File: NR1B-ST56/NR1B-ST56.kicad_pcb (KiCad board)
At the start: 4 copper layers, 70.5 x 134 mm, 34 parts, among them J1 0.1" Female Long Tail, J2 0.1" Female Long Tail, J3 Conn_01x02, U1 S29GL01GP, U2 DG419LDY, U3 OPA2189ID, U4 NCV7800, X1 NUCLEO144-ZIO

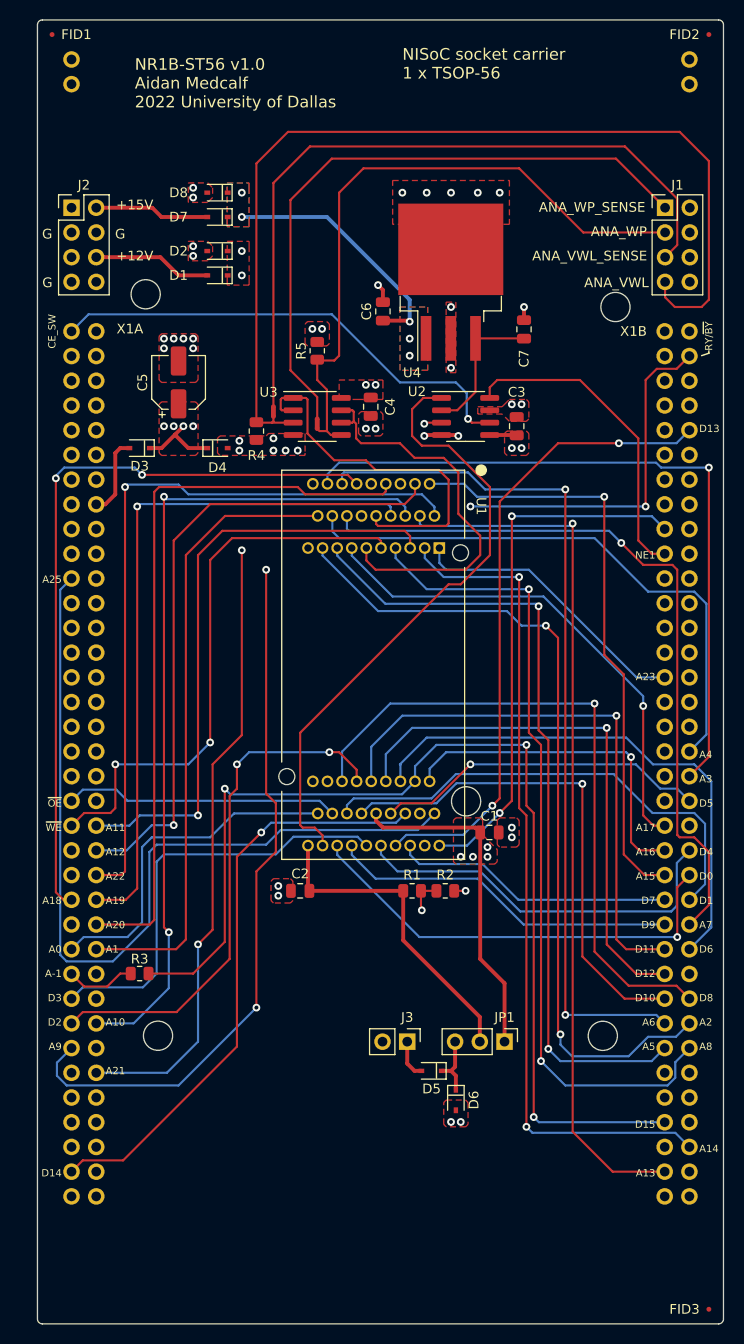
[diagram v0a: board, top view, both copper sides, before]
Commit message: Many updates
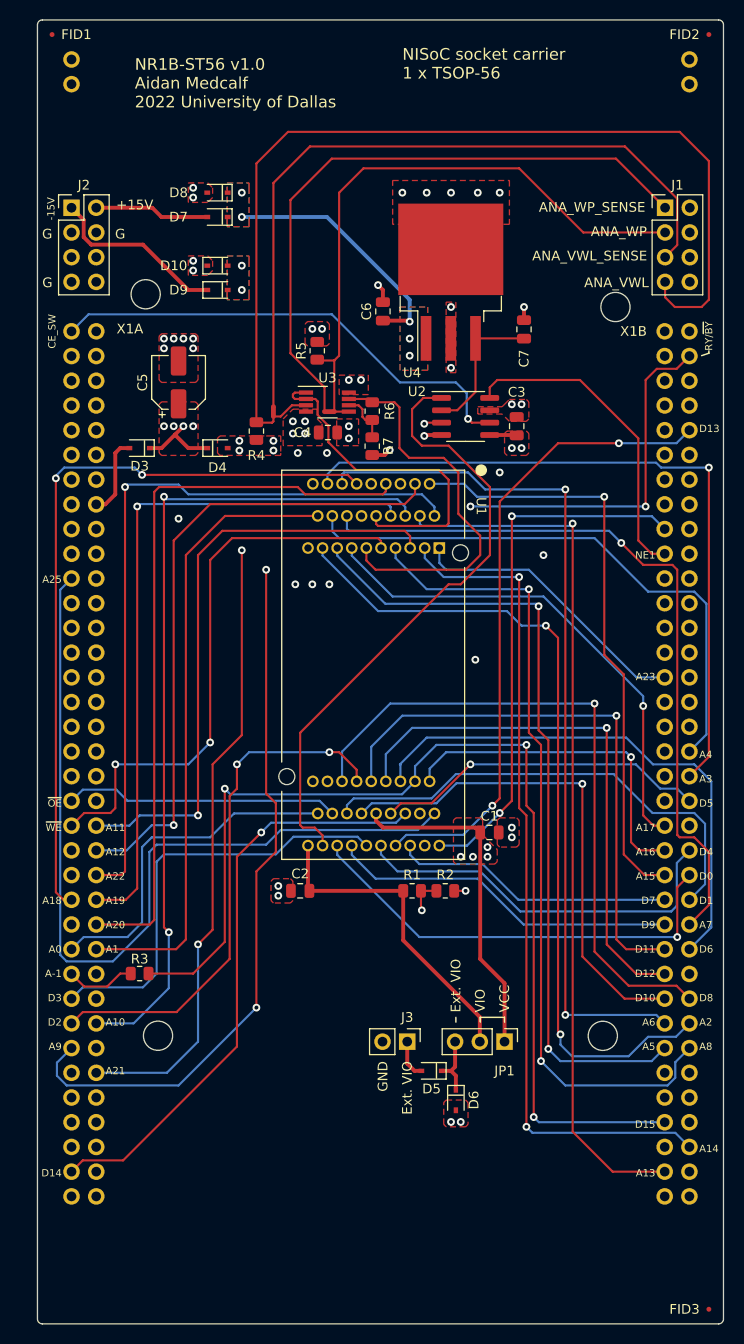
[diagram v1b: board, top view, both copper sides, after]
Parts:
- removed D1: S1G, Diode_SMD:D_SOD-323
- removed D2: 15V, Diode_SMD:D_SOD-323
- added D10: 18V, Diode_SMD:D_SOD-323, F.Cu at (183.5, 104.2)
- added D9: S1G, Diode_SMD:D_SOD-323, F.Cu at (183.5, 106.8)
- added R6: 1K, Resistor_SMD:R_0805_2012Metric, F.Cu at (199.4, 119.2)
- added R7: 1K, Resistor_SMD:R_0805_2012Metric, F.Cu at (199.4, 122.8)
- U3: footprint Package_SO:SOIC-8_3.9x4.9mm_P1.27mm -> Package_SO:VSSOP-8_3.0x3.0mm_P0.65mm
- moved C4 5.14 mm to (194.8, 121.4), turned to 180 degrees
- moved U3 1.81 mm to (194.8, 118.3)
- moved NT2 1.77 mm to (195.0, 119.2), turned to 180 degrees
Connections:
- C4 pad 1: +12V -> +15V
- C4 pad 2: GND -> -15V
- J2 pad 1: unconnected-(J2-Pad1) -> /-15V_IN
- J2 pad 6: /12V_IN -> unconnected-(J2-Pad6)
- U2 pad 4: +12V -> +15V
- U3 pad 4: GND -> -15V
- U3 pad 6: /WP_BUF -> Net-(R6-Pad1)
- U3 pad 8: +12V -> +15V
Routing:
- net +12V: track 24.5 -> 0.00 mm, vias 6 -> 0
- net /-15V_IN: track 0.00 -> 18.5 mm
- net -15V: track 0.00 -> 15.7 mm, vias 0 -> 6
- net /12V_IN: track 12.2 -> 0.00 mm
- net Net-(R6-Pad1): track 0.00 -> 5.27 mm
- net /ANA_WP: track 67.0 -> 63.3 mm
- net /VWL_BUF: track 38.1 -> 36.0 mm
- net GND: track 6.30 -> 8.32 mm, vias 39 -> 45
- net +15V: track 25.8 -> 27.6 mm, vias 5 -> 10
- net /ANA_VWL: track 101.2 -> 102.9 mm
- net /WP_BUF: track 40.9 -> 40.3 mm
- added copper zone on In2.Cu, net +15V
- added copper zone on B.Cu, net -15V
- added copper zone on F.Cu, net -15V
- added copper zone on In2.Cu, net -15V
- removed copper zone on F.Cu, net +12V
- removed copper zone on In2.Cu, net +12V
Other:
- board text added: "-15V"
- board text added: "Ext. VIO"
- board text added: "GND"
- board text added: "VCC"
- board text added: "VIO"
- board text removed: "+12V"
